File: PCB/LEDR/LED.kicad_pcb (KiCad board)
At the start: 2 copper layers, 70 x 70 mm, 47 parts, among them J1 Reset, J2 LED, J3 TC2030-USB-NL-DS, J4 SPK, J5 USB-C-Socket-H, J6 Power, SW1 Button, U1 ICS43434_MEMS_Mic, U2 MAX98357A, U3 Relay, U5 IRM-H638T/TR2, U6 ESP32-S3-MINI-1, U7 MD8942, U8 VEML6040

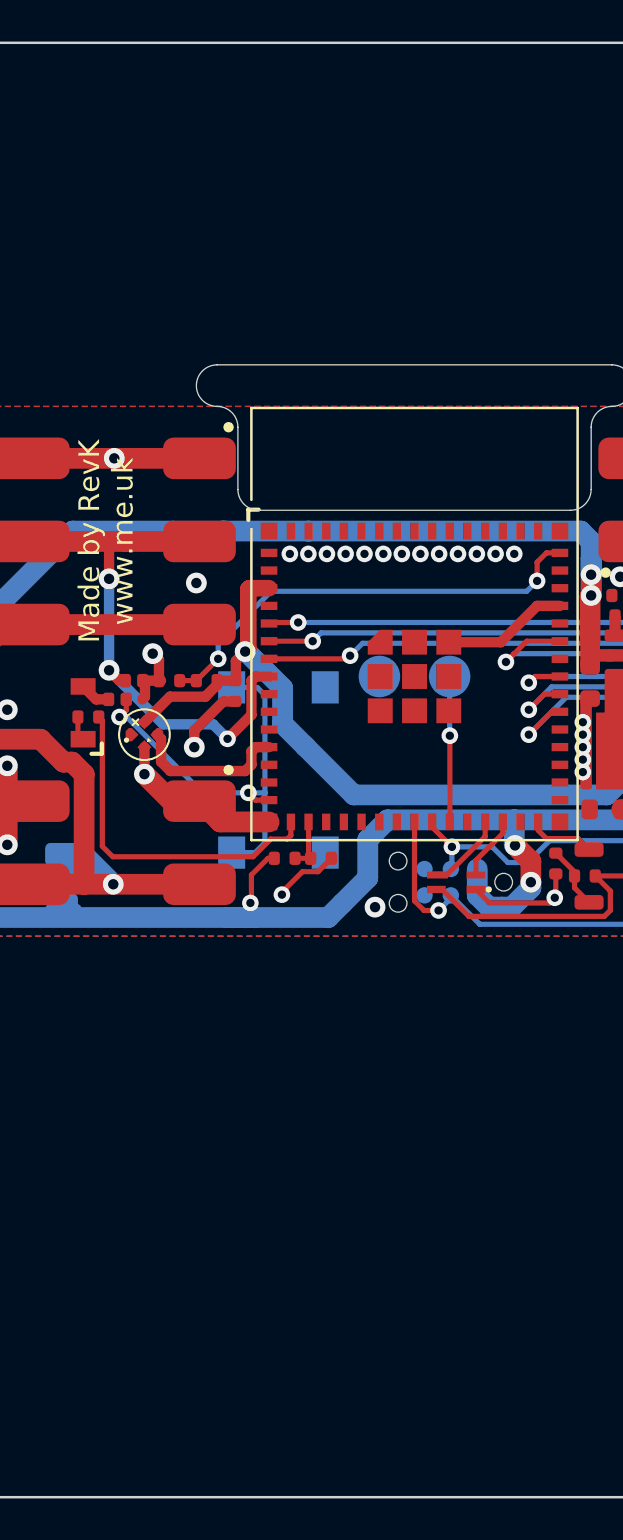
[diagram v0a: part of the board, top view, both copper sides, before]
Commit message: Tidy
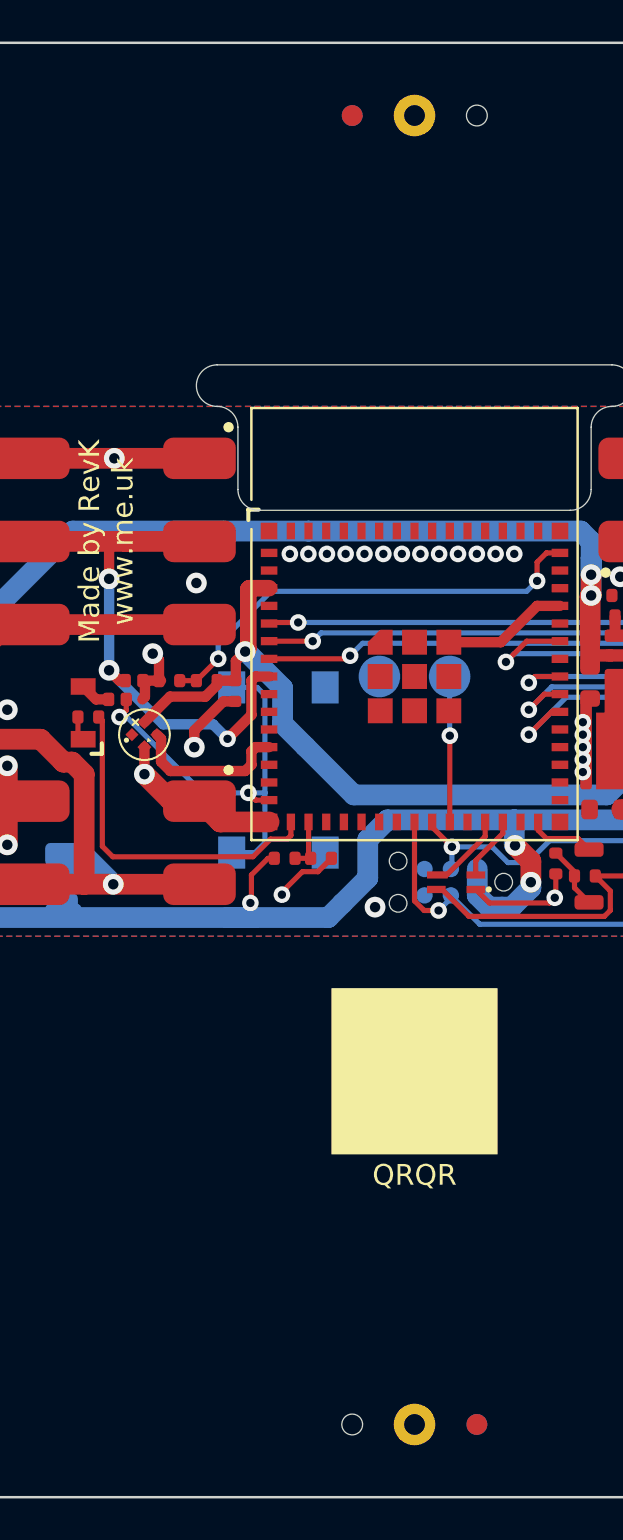
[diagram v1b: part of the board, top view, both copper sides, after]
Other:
- board text added: "QRQR"
